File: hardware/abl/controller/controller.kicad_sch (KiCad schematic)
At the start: 36 parts, among them IC1 TCA6408ARSVR, IC2 TCA6408ARSVR, IC3 VEML6040A3OG, IC4 TXB0104RUT, J1 SFW20S-2STE1LF, J2 Conn_02x05_Odd_Even, J3 Conn_02x05_Odd_Even, J4 PRT-14417, J5 Conn_02x05_Odd_Even, J6 Conn_01x10_Pin, J7 Conn_01x10_Pin, J8 Conn_01x16, J9 Conn_01x12, Q2 AO3401A, Q4 AO3401A

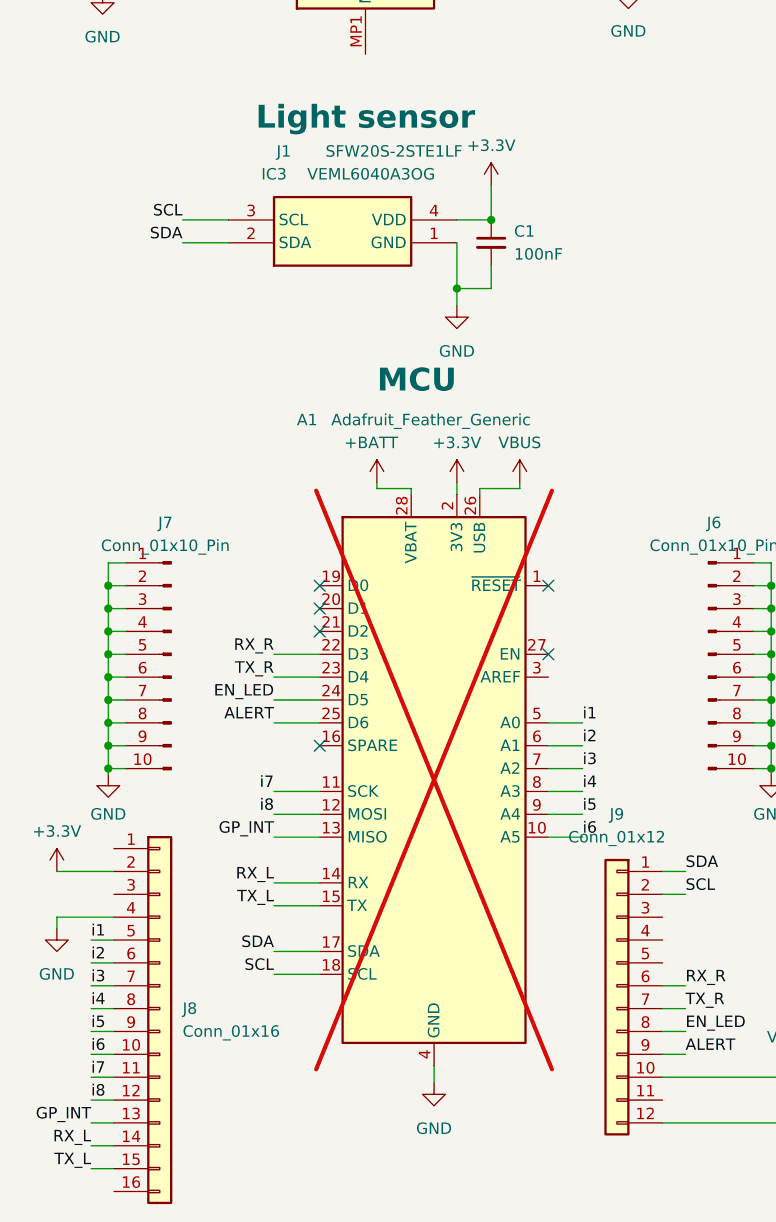
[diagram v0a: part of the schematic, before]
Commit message: Even more small adjustments before ordering v1.2 of controller module.
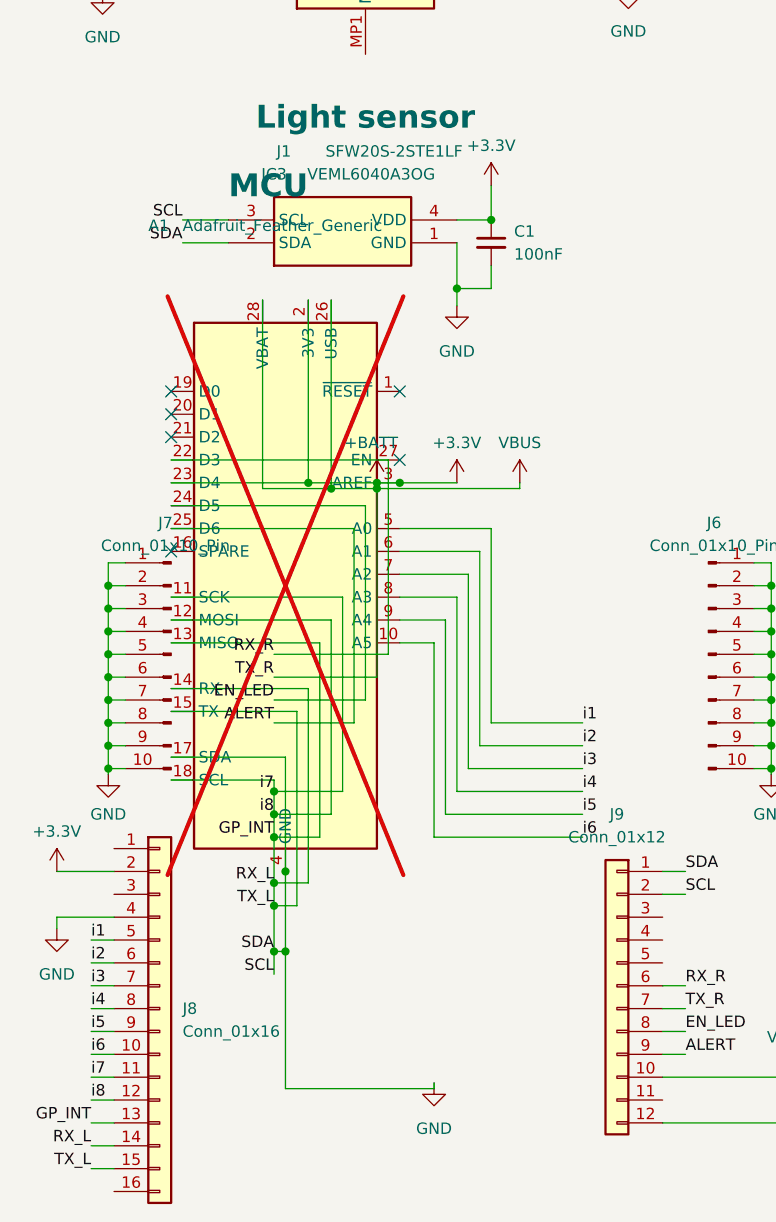
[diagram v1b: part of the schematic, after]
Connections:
- net +5V is gone; now on net +3.3V: A1.28 (VBAT), C12.1, C8.2, D1.1 (K), IC2.14 (VCCP), IC4.11 (VCCB), J1.16, J1.19, J1.8, J5.4 (Pin_4), J5.6 (Pin_6), J9.12 (Pin_12), Q2.2 (S), Q4.2 (S), TP3.1
- net GP_INT is gone; now on net GND: A1.13 (MISO), IC1.11 (~{INT}), IC2.11 (~{INT}), J8.13 (Pin_13)
- net RX_L is gone; now on net GND: A1.14 (RX), IC4.3 (A2), J2.7 (Pin_7), J8.14 (Pin_14)
- net SCL is gone; now on net GND: A1.18 (SCL), IC1.12 (SCL), IC2.12 (SCL), IC3.3 (SCL), J1.3, J4.4, J5.3 (Pin_3), J9.2 (Pin_2), R4.2
- net SDA is gone; now on net GND: A1.17 (SDA), IC1.13 (SDA), IC2.13 (SDA), IC3.2 (SDA), J1.1, J4.3, J5.1 (Pin_1), J9.1 (Pin_1), R5.1
- net TX_L is gone; now on net GND: A1.15 (TX), IC4.2 (A1), J2.9 (Pin_9), J8.15 (Pin_15)
- net TX_R is gone; now on net +3.3V: A1.23 (D4), IC4.4 (A3), J3.9 (Pin_9), J9.7 (Pin_7)
- net VBUS is gone; now on net +3.3V: A1.26 (USB), D1.2 (A), J9.10 (Pin_10)
- net i7 is gone; now on net GND: A1.11 (SCK), J1.11, J8.11 (Pin_11)
- net i8 is gone; now on net GND: A1.12 (MOSI), J1.9, J8.12 (Pin_12)
- net +3.3V: now also A1.3 (AREF)
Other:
- moved on the sheet: A1
